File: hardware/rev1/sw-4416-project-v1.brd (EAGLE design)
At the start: 94 x 53.3 mm, 57 parts, among them IC1 MCP73831, U1 ADP3338, X1 USB-MICROB, Y1 16M

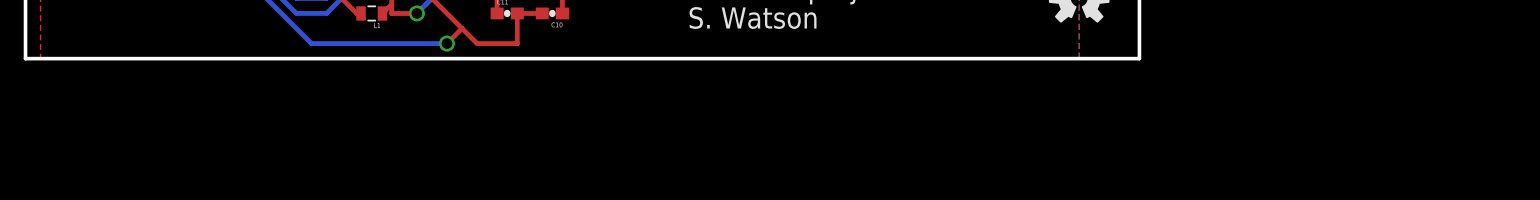
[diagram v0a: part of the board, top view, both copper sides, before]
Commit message: open sourcing hardware and software
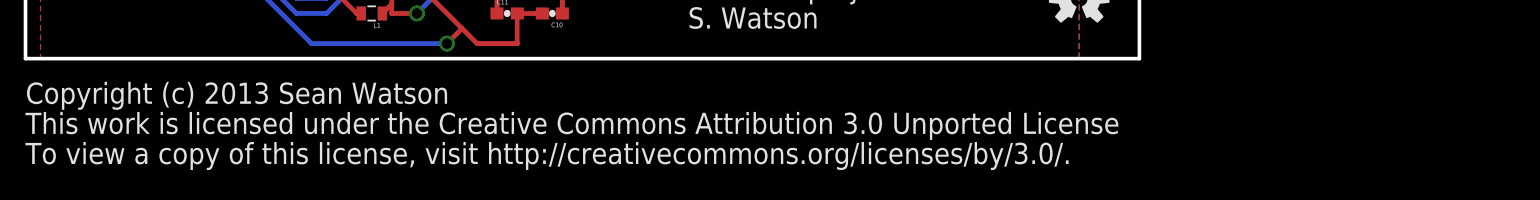
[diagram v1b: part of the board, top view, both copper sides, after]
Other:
- board text added: "Copyright (c) 2013 Sean Watson"
- board text added: "This work is licensed under the Creative Commons Attribution 3.0 Unported License"
- board text added: "To view a copy of this license, visit http://creativecommons.org/licenses/by/3.0/."
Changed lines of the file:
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@@
 <dimension x1="93.98" y1="78.74" x2="0" y2="78.74" x3="46.99" y3="85.09" layer="51"/>
 <dimension x1="93.98" y1="78.74" x2="93.98" y2="26.67" x3="104.14" y3="52.705" layer="51"/>
+<text x="0" y="22.86" size="1.778" layer="25">Copyright (c) 2013 Sean Watson</text>
+<text x="0" y="20.32" size="1.778" layer="25">This work is licensed under the Creative Commons Attribution 3.0 Unported License</text>
+<text x="0" y="17.78" size="1.778" layer="25">To view a copy of this license, visit http://creativecommons.org/licenses/by/3.0/.</text>
 </plain>
 <attributes>
